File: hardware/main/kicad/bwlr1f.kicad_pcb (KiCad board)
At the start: 4 copper layers, 61.2 x 26.1 mm, 61 parts, among them J1 Conn_01x02, U1 RAK3172-SIP, U2 NBM7100ABQX, U3 ZD24C08A, U4 BME688, U5 RV-3028-C7

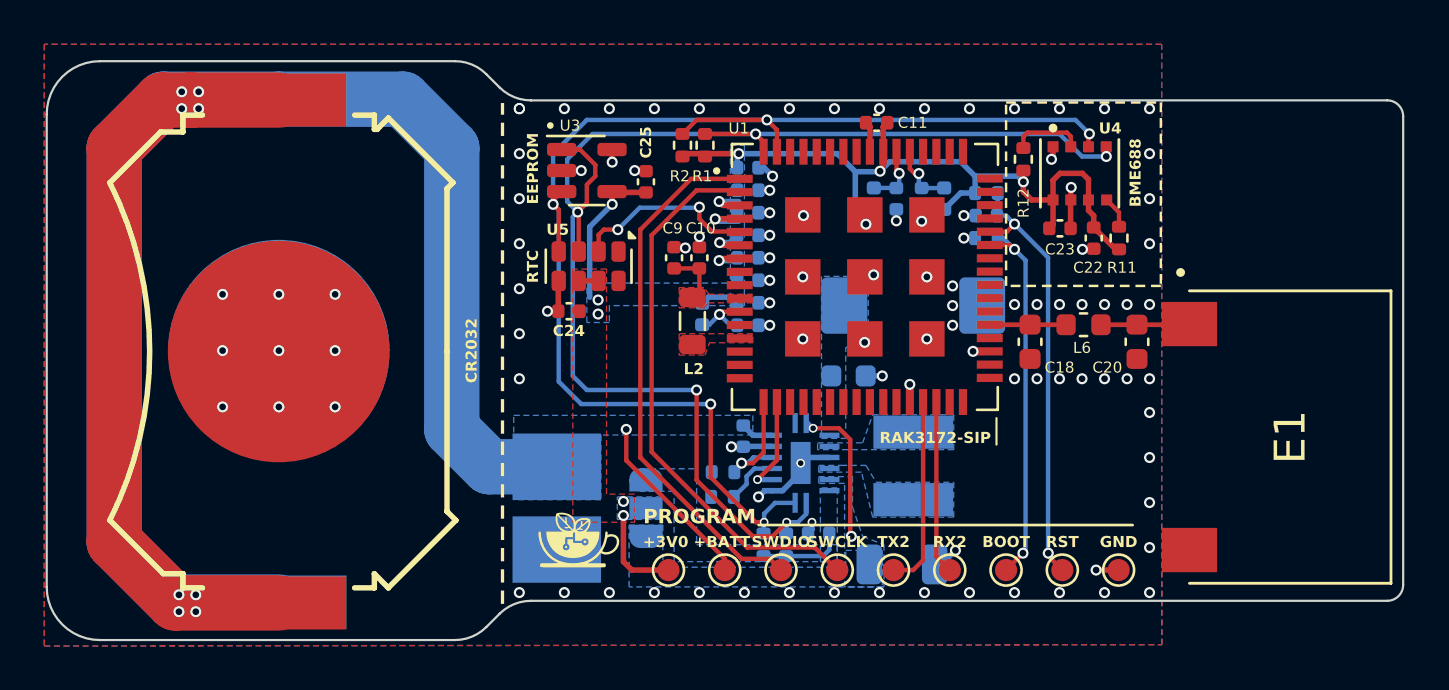
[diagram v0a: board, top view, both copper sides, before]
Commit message: Update Programmer
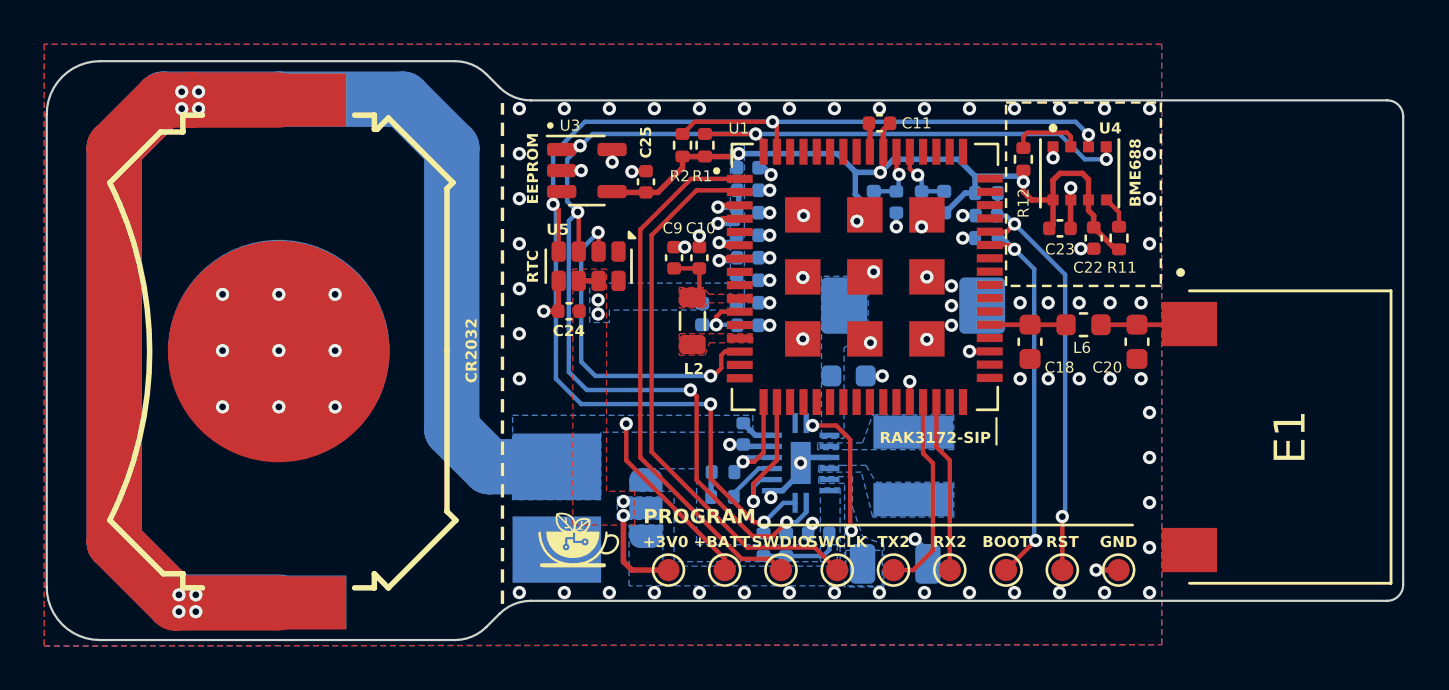
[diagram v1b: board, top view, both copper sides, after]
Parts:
- moved C21 0.31 mm to (143.8, 120.2)
- moved C12 0.15 mm to (143.8, 103.8)
- moved C13 0.15 mm to (145.0, 103.8)
- moved L3 0.15 mm to (142.8, 103.8)
- moved L4 0.15 mm to (146.0, 103.8)
- moved C11 0.13 mm to (143.1, 100.3)
- moved C15 0.10 mm to (136.9, 114.3)
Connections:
- U1 pad 14: unconnected-(U1-PB3-Pad14) -> /RTC_WKUP
- U1 pad 5: /RTC_WKUP -> unconnected-(U1-PC13-Pad5)
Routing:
- net /RTC_WKUP: track 8.42 -> 15.2 mm
- net /SCL: track 62.4 -> 59.1 mm, vias 5 -> 6
- net +3V0: track 56.1 -> 53.1 mm, vias 12 -> 11
- net GND: track 27.2 -> 29.3 mm, vias 108 -> 103
- net /RDY: track 4.51 -> 6.55 mm
